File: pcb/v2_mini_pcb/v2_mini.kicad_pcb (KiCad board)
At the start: 6 copper layers, 60.8 x 35.1 mm, 113 parts, among them J1 Conn_Coaxial, J2 GTFP08441BEU, J3 SFV24R-2STE1HLF, J5 TC2030, J6 USB4105-GF-A, Q1 NTNS3164NZT5G, SW1 SW_Push, SW2 SW_Push, SW3 SW_Push, SW4 SW_Push, SW5 SW_Push, SW6 SW_Push, U1 UM980, U10 TPS63802DLAR, U3 SCH16T-K01-1, U4 LP5813ADRRR, U5 TCA9536ADTMR, U6 TPD4EUSB30, U8 BQ25622ERYKR, U9 MAX17048G_T10

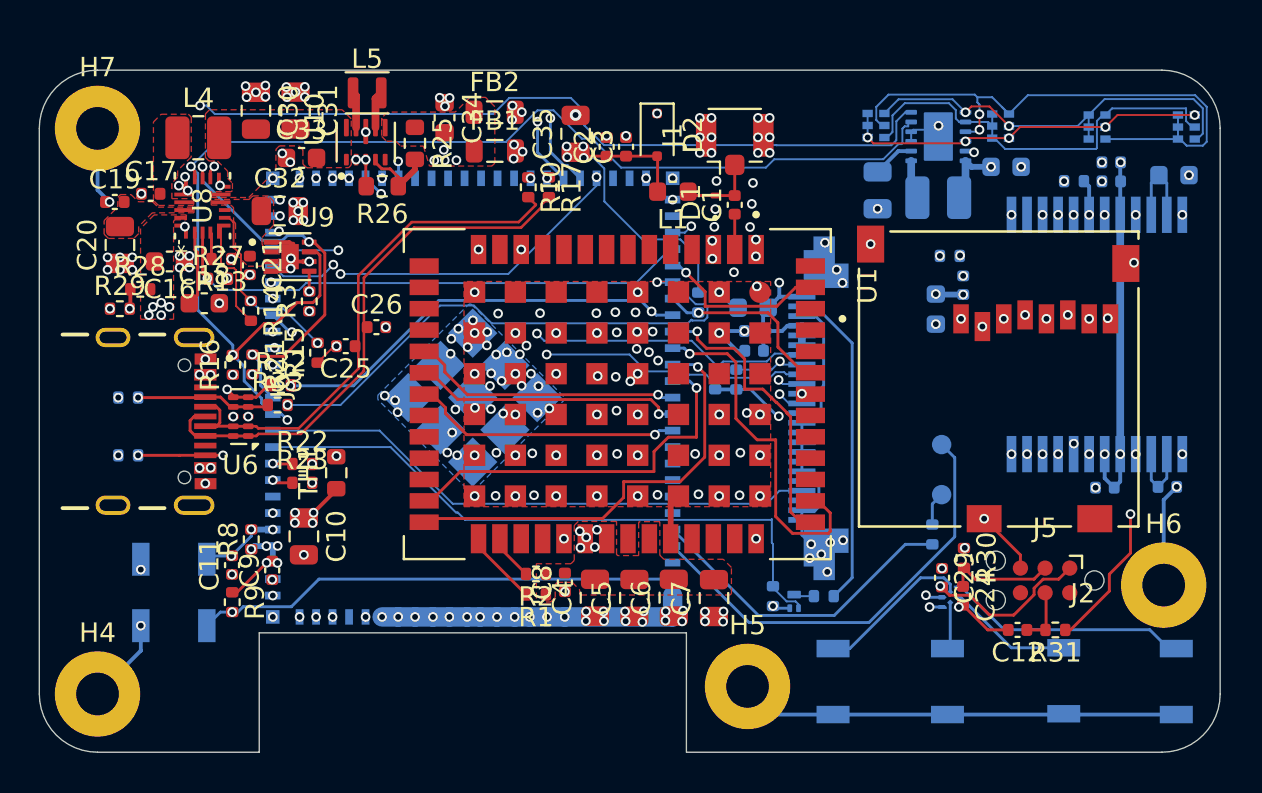
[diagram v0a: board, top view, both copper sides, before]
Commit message: draw
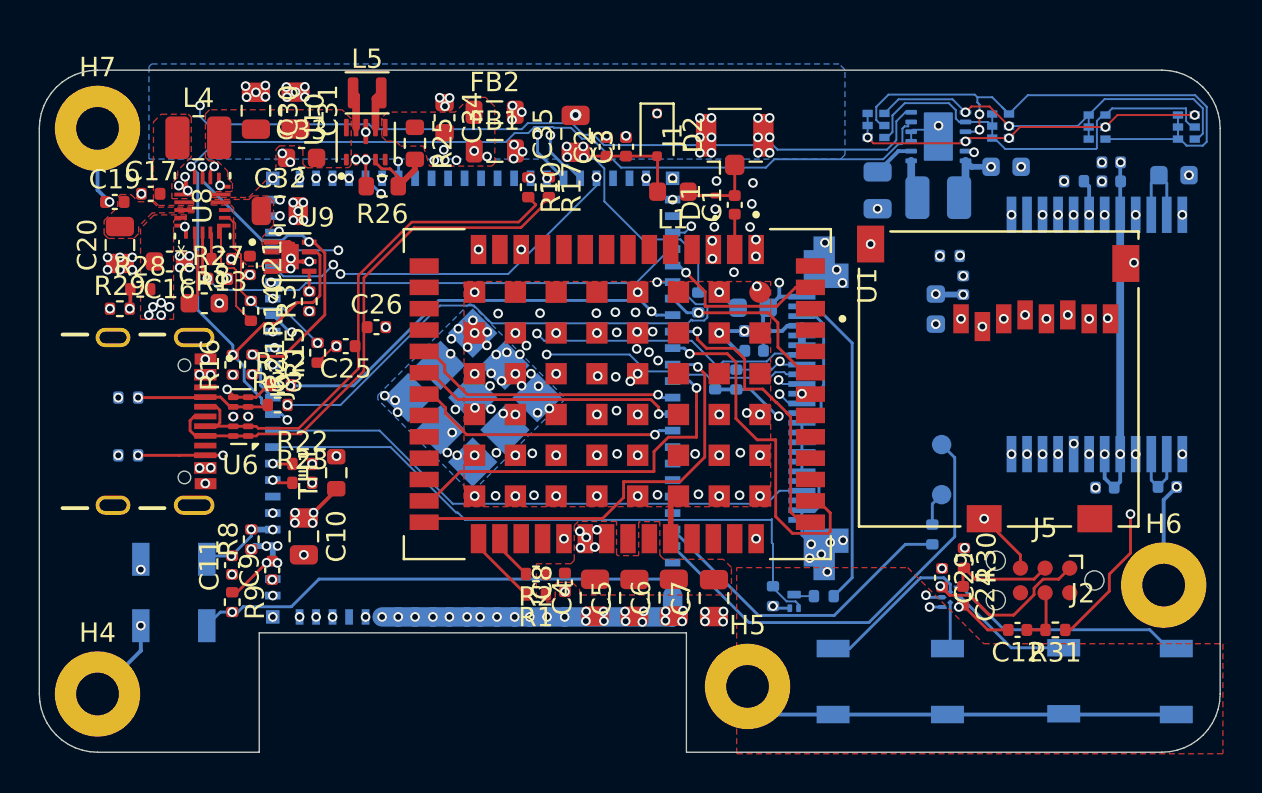
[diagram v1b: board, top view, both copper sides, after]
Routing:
- net +3V3: track 143.7 -> 56.9 mm, vias 23 -> 25
- net /ESP32-S31 MCU/POW_SCL: track 103.3 -> 102.6 mm
- added copper zone on In3.Cu, net GND
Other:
- outline, holes or cut-outs redrawn
- board text added: "gh/teehee567"
